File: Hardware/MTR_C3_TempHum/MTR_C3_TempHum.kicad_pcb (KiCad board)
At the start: 4 copper layers, 87.6 x 24.1 mm, 62 parts, among them IC1 ESP32-C3-MINI-1-H4, IC2 BQ25170DSGR, IC3 BH1750FVI-TR, IC4 DHT22, IC5 RT9080-33GJ5, J1 Korean Hroparts Elec TYPE-C-3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, J2 Boot Option, J4 B5B-XH-A_LF__SN_, Q3 AO3401A, Q5 AO3402, Q6 AO3401A, Q7 AO3402, SW1 Reset, SW2 Hard_reset

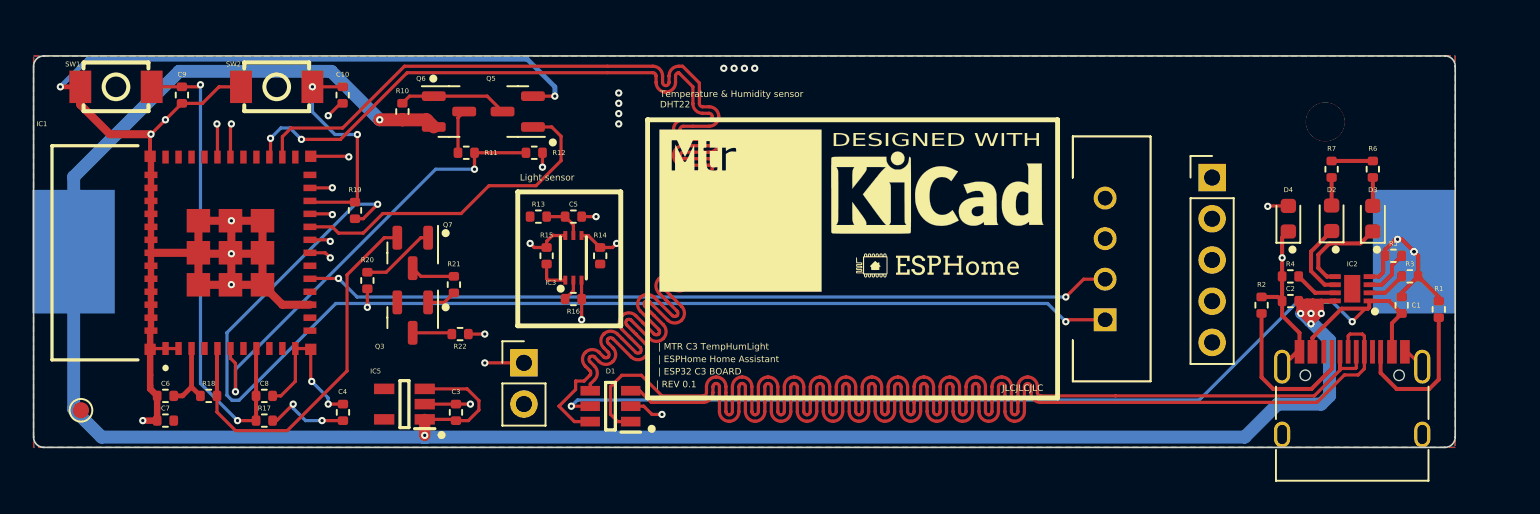
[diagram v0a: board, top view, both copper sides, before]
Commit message: V0.2.0
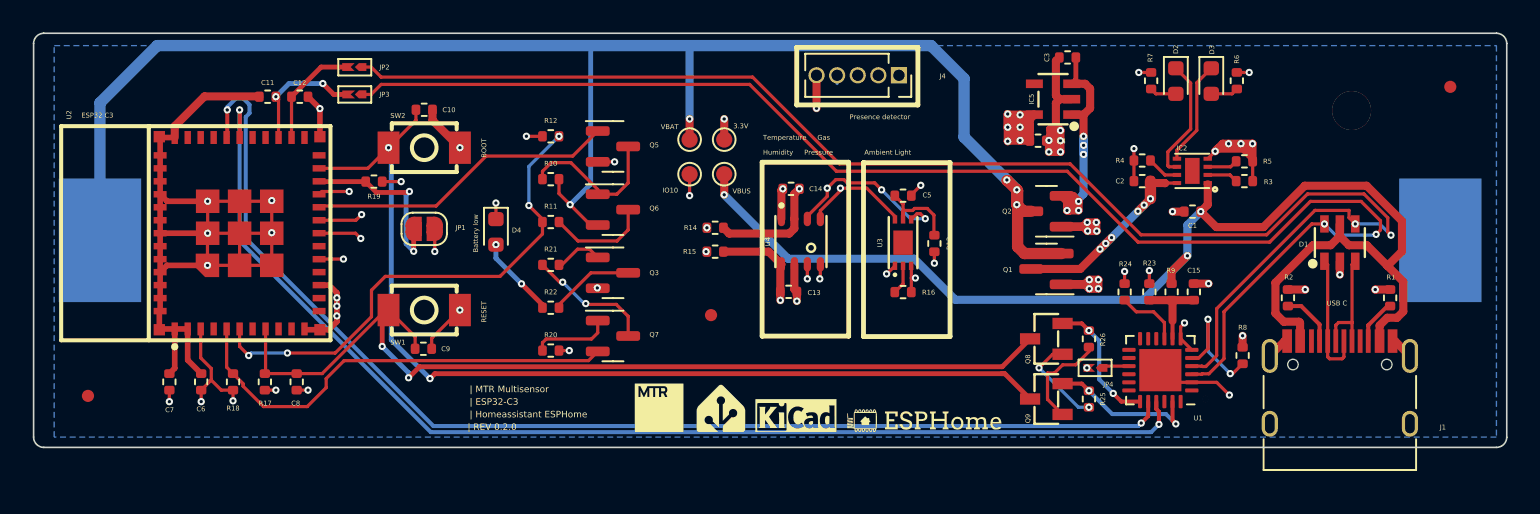
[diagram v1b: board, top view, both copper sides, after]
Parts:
- removed ? (x9): , clipboard:4e852f44-b39c-41c1-9906-6824c0cbc5c7
- removed ?: , clipboard:907f2ce9-957e-4633-84d2-7c9ab30228eb
- removed the G*** at (81.7, 36.8)
- removed IC1: ESP32-C3-MINI-1-H4, SamacSys_Parts:ESP32C3MINI1H4
- removed IC3: BH1750FVI-TR, SamacSys_Parts:WSOF6
- removed IC4: DHT22, SamacSys_Parts:DHT22
- removed J2: Boot Option, PinHeader:PinHeader_1x02_P2.54mm_Vertical
- removed REF**: LOGO, Library:KiCad
- added C11: 22p, Resistor_SMD:R_0402_1005Metric, F.Cu at (52.5, 29.8)
- added C12: 22p, Resistor_SMD:R_0402_1005Metric, F.Cu at (54.5, 29.8)
- added C13: 100n, Resistor_SMD:R_0402_1005Metric, F.Cu at (84.6, 41.8)
- added C14: 100n, Resistor_SMD:R_0402_1005Metric, F.Cu at (84.8, 35.5)
- added C15: 1u, Resistor_SMD:R_0402_1005Metric, F.Cu at (109.6, 41.8)
- added FID1: Fiducial, Fiducial:Fiducial_0.75mm_Mask2.25mm, F.Cu at (41.5, 48.3)
- added FID2: Fiducial, Fiducial:Fiducial_0.75mm_Mask2.25mm, F.Cu at (79.9, 43.3)
- added FID3: Fiducial, Fiducial:Fiducial_0.75mm_Mask2.25mm, F.Cu at (125.4, 29.2)
- added G***: LOGO, LOGO, F.Cu at (80.5, 49.0)
- added G***: LOGO, LOGO, F.Cu at (85.1, 49.5)
- added G***: LOGO, LOGO, F.Cu at (76.7, 49.0)
- added G***: LOGO, LOGO, F.Cu at (93.1, 49.8)
- added JP1: Soft_reset, Jumper:SolderJumper-2_P1.3mm_Open_RoundedPad1.0x1.5mm, F.Cu at (62.2, 38.0)
- added JP2: D-, Jumper:SolderJumper-2_P1.3mm_Open_TrianglePad1.0x1.5mm, F.Cu at (57.9, 28.0)
- added JP3: D+, Jumper:jumper perso1, F.Cu at (57.9, 29.7)
- added JP4: SUSPEND, Jumper:SolderJumper-2_P1.3mm_Open_TrianglePad1.0x1.5mm, F.Cu at (103.5, 46.5)
- added Q1: AO3401A, Package_TO_SOT_SMD:SOT-23, F.Cu at (100.5, 40.4)
- added Q2: AO3401A, Package_TO_SOT_SMD:SOT-23, F.Cu at (100.5, 36.9)
- added Q8: S8050, easyeda2kicad:SOT-23-3_L2.9-W1.3-P1.90-LS2.4-BR, F.Cu at (100.5, 44.7)
- added Q9: S8050, easyeda2kicad:SOT-23-3_L2.9-W1.3-P1.90-LS2.4-BR, F.Cu at (100.5, 48.5)
- added R23: 47k5, Resistor_SMD:R_0402_1005Metric, F.Cu at (106.9, 41.8)
- added R24: 1k, Resistor_SMD:R_0402_1005Metric, F.Cu at (105.4, 41.8)
- added R25: 10k, Resistor_SMD:R_0402_1005Metric, F.Cu at (103.2, 48.5)
- added R26: 10k, Resistor_SMD:R_0402_1005Metric, F.Cu at (103.2, 44.7)
- added R8: 1k, Resistor_SMD:R_0402_1005Metric, F.Cu at (112.6, 45.8)
- added R9: 22k1, Resistor_SMD:R_0402_1005Metric, F.Cu at (108.2, 41.8)
- added TP2: TestPoint, TestPoint:TestPoint_Pad_D1.0mm, F.Cu at (80.7, 32.5)
- added TP3: TestPoint, TestPoint:TestPoint_Pad_D1.0mm, F.Cu at (80.7, 34.6)
- added TP4: TestPoint, TestPoint:TestPoint_Pad_D1.0mm, F.Cu at (78.5, 34.6)
- added U1: CP2102N-Axx-xQFN24, Package_DFN_QFN:QFN-24-1EP_4x4mm_P0.5mm_EP2.6x2.6mm, F.Cu at (107.6, 46.7)
- added U2: ESP32-C3-MINI-1-H4(4MB), easyeda2kicad:WIFIM-SMD_ESP32-C3-MINI-1, F.Cu at (50.8, 38.2)
- added U3: BH1750FVI-TR, easyeda2kicad:WSOF-6_L2.6-W1.6-P0.50-TL-EP, F.Cu at (91.7, 38.8)
- added U4: BME680, easyeda2kicad:LGA-8_L3.0-W3.0-P0.80-TR, F.Cu at (85.4, 38.8)
- D1: footprint SamacSys_Parts:SOT95P280X145-6N -> easyeda2kicad:SOT-23-6_L2.9-W1.6-P0.95-LS2.8-BL
- IC2: footprint SamacSys_Parts:SON50P200X200X80-9N -> easyeda2kicad:WSON-8_L2.0-W2.0-P0.50-TL-EP
- IC5: footprint SamacSys_Parts:SOT94P280X100-5N -> easyeda2kicad:TSOT-23-5_L2.9-W1.6-P0.95-LS2.8-BL
- J4: footprint PinHeader:PinHeader_1x05_P2.54mm_Vertical -> Connector_PinSocket_1.27mm:PinSocket_1x05_P1.27mm_Vertical
- SW2: value Hard_reset -> Boot
- moved D4 48.9 mm to (66.6, 38.2), turned to -90 degrees
- moved D1 46.1 mm to (118.6, 38.8), turned to 0 degrees
- moved C4 46.0 mm to (100.0, 32.5), turned to 180 degrees
- moved IC5 44.2 mm to (100.9, 30.0), turned to 90 degrees
- moved C3 43.6 mm to (101.8, 27.4), turned to 0 degrees
- moved TP1 41.1 mm to (78.5, 32.5)
- moved R13 24.5 mm to (93.6, 38.9), turned to -90 degrees
- moved SW1 23.5 mm to (62.2, 43.0), turned to 180 degrees
- moved C9 21.6 mm to (62.1, 45.4), turned to 180 degrees
- moved C5 20.4 mm to (91.7, 35.9)
- moved R16 20.3 mm to (91.7, 41.9)
- moved J4 20.3 mm to (91.4, 28.5), turned to -90 degrees
- moved C1 14.1 mm to (109.5, 36.9), turned to 0 degrees
- moved Q7 13.4 mm to (73.8, 44.6), turned to 0 degrees
- moved D3 13.1 mm to (110.7, 28.9), turned to -90 degrees
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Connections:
- net EN renamed CHIP_PU
- C10 pad 2: Hard_reset -> GPIO9
- C2 pad 1: VBAT -> Net-(IC2-OUT)
- C3 pad 2: VBAT -> Net-(IC5-EN)
- IC2 pad 8: VBAT -> Net-(IC2-OUT)
- IC5 pad 1: VBAT -> Net-(IC5-EN)
- IC5 pad 3: VBAT -> Net-(IC5-EN)
- J4 pad 2: UART_RX -> U0RXD
- J4 pad 3: UART_TX -> U0TXD
- SW2 pad 2: Hard_reset -> GPIO9
- TP1 pad 1: +3.3V -> VBAT
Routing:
- net U0RXD: track 0.00 -> 114.6 mm, vias 0 -> 2
- net U0TXD: track 0.00 -> 114.1 mm, vias 0 -> 2
- net /D-: track 102.2 -> 8.05 mm
- net /D+: track 98.9 -> 7.05 mm
- net +3.3V: track 126.1 -> 50.7 mm, vias 13 -> 25
- net UART_TX: track 68.8 -> 0.00 mm, vias 1 -> 0
- net UART_RX: track 64.9 -> 0.00 mm, vias 1 -> 0
- net VBAT: track 154.5 -> 102.6 mm, vias 6 -> 5
- net DHT22_DATA: track 50.0 -> 0.00 mm, vias 2 -> 0
- net Net-(D4-A): track 53.8 -> 5.08 mm
- net GPIO9: track 18.5 -> 60.9 mm
- net CHIP_PU: track 30.3 -> 59.4 mm
- net GPIO10: track 0.00 -> 27.2 mm, vias 0 -> 2
- net SCL: track 16.5 -> 41.5 mm, vias 2 -> 3
- net SDA: track 22.2 -> 44.8 mm, vias 2 -> 5
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- added copper zone on In1.Cu, net +3.3V
- removed copper zone on F.Cu, net +3.3V
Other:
- board size 87.6 x 24.1 mm -> 90.8 x 25.5 mm
- board text added: "3.3V"
- board text added: "Ambient Light"
- board text added: "BOOT"
- board text added: "Battery low"
- board text added: "ESP32 C3"
- board text added: "Gas"
- board text added: "Humidity"
- board text added: "IO10"
- board text added: "Presence detector"
- board text added: "Pressure"
- board text added: "RESET"
- board text added: "Temperature"
- board text added: "USB C"
- board text added: "VBAT"
- board text added: "VBUS"
- board text added: "| ESP32-C3"
- board text added: "| Homeassistant ESPHome"
- board text added: "| MTR Multisensor"
- board text added: "| REV 0.2.0"
- board text removed: "JLCJLCJLC"
- board text removed: "Light sensor"
- board text removed: "Temperature & Humidity sensor DHT22"
- board text removed: "| ESP32 C3 BOARD"
- board text removed: "| ESPHome Home Assistant"
- board text removed: "| MTR C3 TempHumLight"
- board text removed: "| REV 0.1"
